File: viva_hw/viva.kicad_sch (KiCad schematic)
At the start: 35 parts, among them J1 Motor, J2 Measure_enable, J3 Battery_in, J4 OLED, J5 Battery_out, M1 XIAO_ESP32C3, Q1 NMOS, Q2 NMOS, Q3 NMOS, Q4 NMOS, SW1 SW_DPDT_x2, SW2 SW_DPST_x2, SW3 SW_DPST_x2

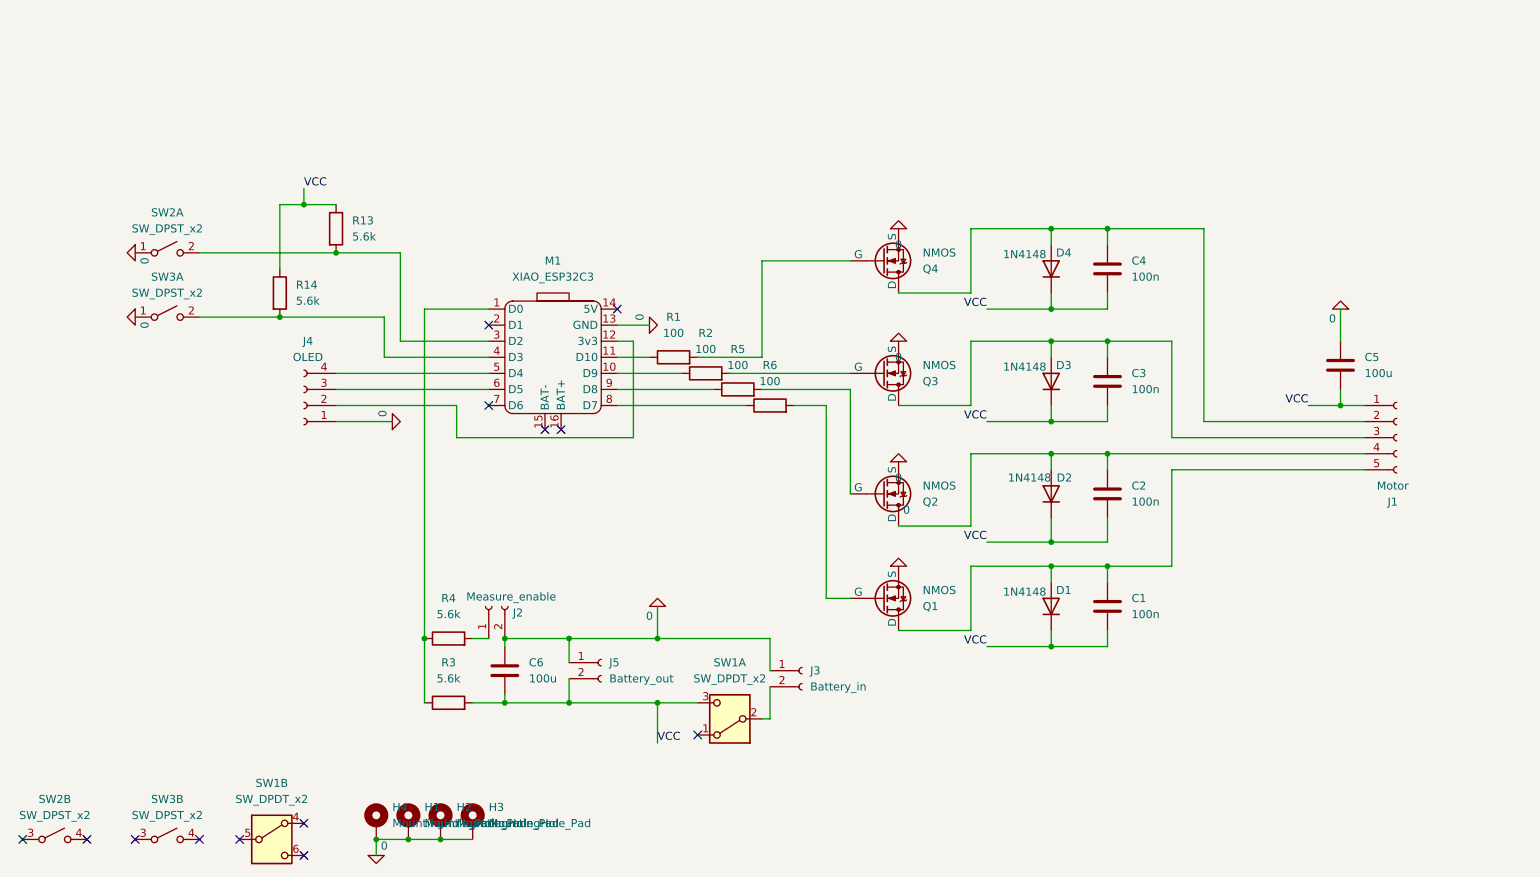
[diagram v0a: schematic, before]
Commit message: feat: v2, changed controller
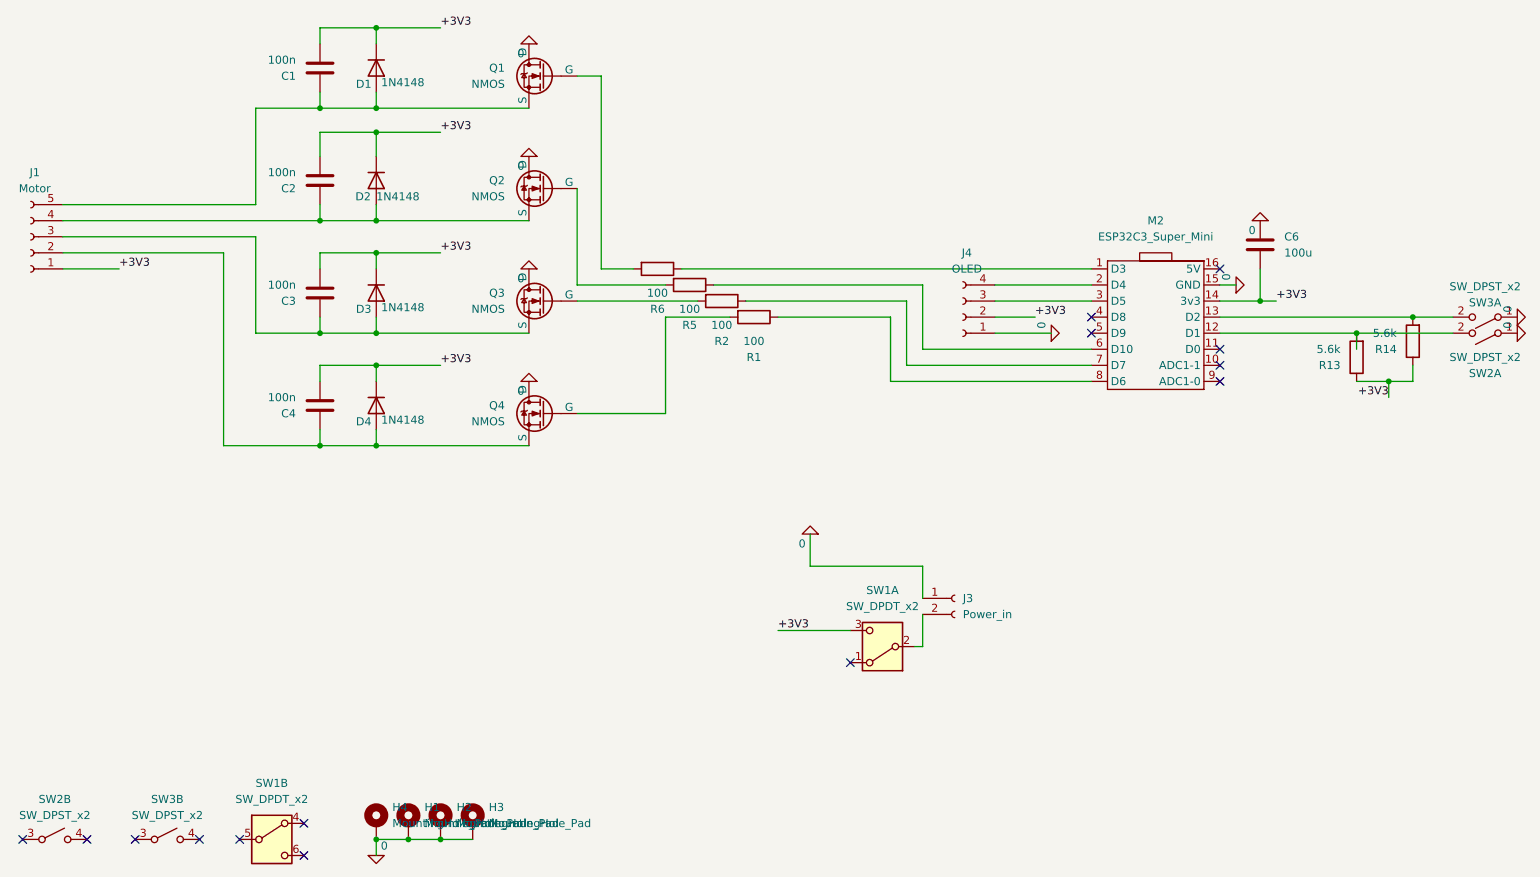
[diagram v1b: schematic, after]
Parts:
- removed C5: 100u, Capacitor_THT:CP_Radial_D8.0mm_P3.50mm, symbol Device:C
- removed J2: Measure_enable, Connector_PinHeader_2.54mm:PinHeader_1x02_P2.54mm_Vertical, symbol Connector:Conn_01x02_Socket
- removed J5: Battery_out, Connector_PinHeader_2.00mm:PinHeader_1x02_P2.00mm_Vertical, symbol Connector:Conn_01x02_Socket
- removed M1: XIAO_ESP32C3, System_On_Chip:XIAO_ESP32C3_THR, symbol System_On_Chip:XIAO_ESP32C3
- removed R3, R4: 5.6k, Resistor_THT:R_Axial_DIN0207_L6.3mm_D2.5mm_P10.16mm_Horizontal, symbol Device:R
- added M2: ESP32C3_Super_Mini, System_On_Chip:ESP32C3_SUPER_MINI_THR, symbol System_On_Chip:ESP32C3_Super_Mini
- J3: value Battery_in -> Power_in; footprint Connector_PinHeader_2.00mm:PinHeader_1x02_P2.00mm_Vertical -> Additional_Connectors:Barrel_Plug_5.5mmx2.1mm
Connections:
- net VCC is gone; now on net +3V3: C1.1, C2.1, C3.1, C4.1, C6.1, D1.1 (K), D2.1 (K), D3.1 (K), D4.1 (K), J1.1 (Pin_1), R13.1, R14.1, SW1.3 (C)
- net 0: now also Q1.1 (D), Q2.1 (D), Q3.1 (D), Q4.1 (D), M2.15 (GND); no longer Q1.3 (S), Q2.3 (S), Q3.3 (S), Q4.3 (S)
- net at C4.2, D4.2 (A), J1.2 (Pin_2): now also Q4.3 (S); no longer Q4.1 (D)
- net at C2.2, D2.2 (A), J1.4 (Pin_4): now also Q2.3 (S); no longer Q2.1 (D)
- net at R14.2, SW3.2 (B): now also M2.13 (D2)
- net at R6.1: now also M2.1 (D3)
- net at C3.2, D3.2 (A), J1.3 (Pin_3): now also Q3.3 (S); no longer Q3.1 (D)
- net at C1.2, D1.2 (A), J1.5 (Pin_5): now also Q1.3 (S); no longer Q1.1 (D)
- net at R1.1: now also M2.8 (D6)
- net +3V3: now reaches J4.2 (Pin_2)
- net +3V3: now also M2.14 (3v3)
- net at J4.3 (Pin_3): now also M2.3 (D5)
- net at J4.4 (Pin_4): now also M2.2 (D4)
- net at R13.2, SW2.2 (B): now also M2.12 (D1)
- net at R2.1: now also M2.7 (D7)
- net at R5.1: now also M2.6 (D10)
- no-connect marks 13 -> 14
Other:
- moved on the sheet: C1, C2, C3, C4, C6, D1, D2, D3, D4, J1, J3, J4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
